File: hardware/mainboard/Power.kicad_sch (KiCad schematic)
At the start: 49 parts, among them IC1 3.3V/0.5A, IC2 TPS54202HDDCR, U12 LMR33640DDDA

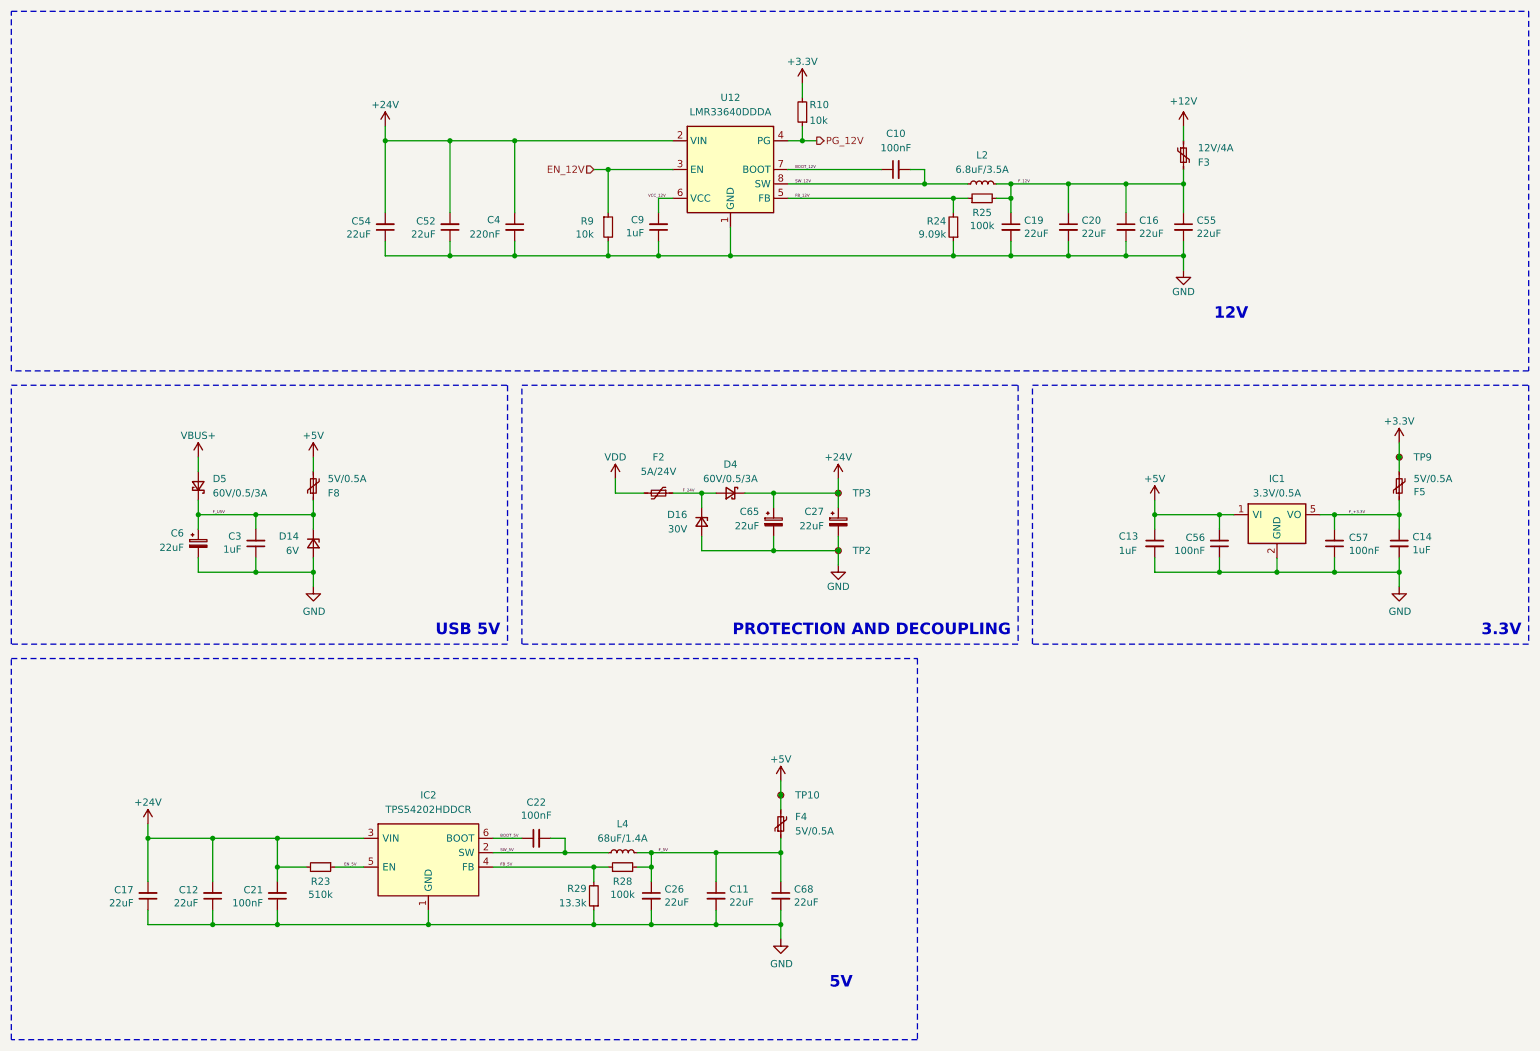
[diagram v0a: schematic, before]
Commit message: sync
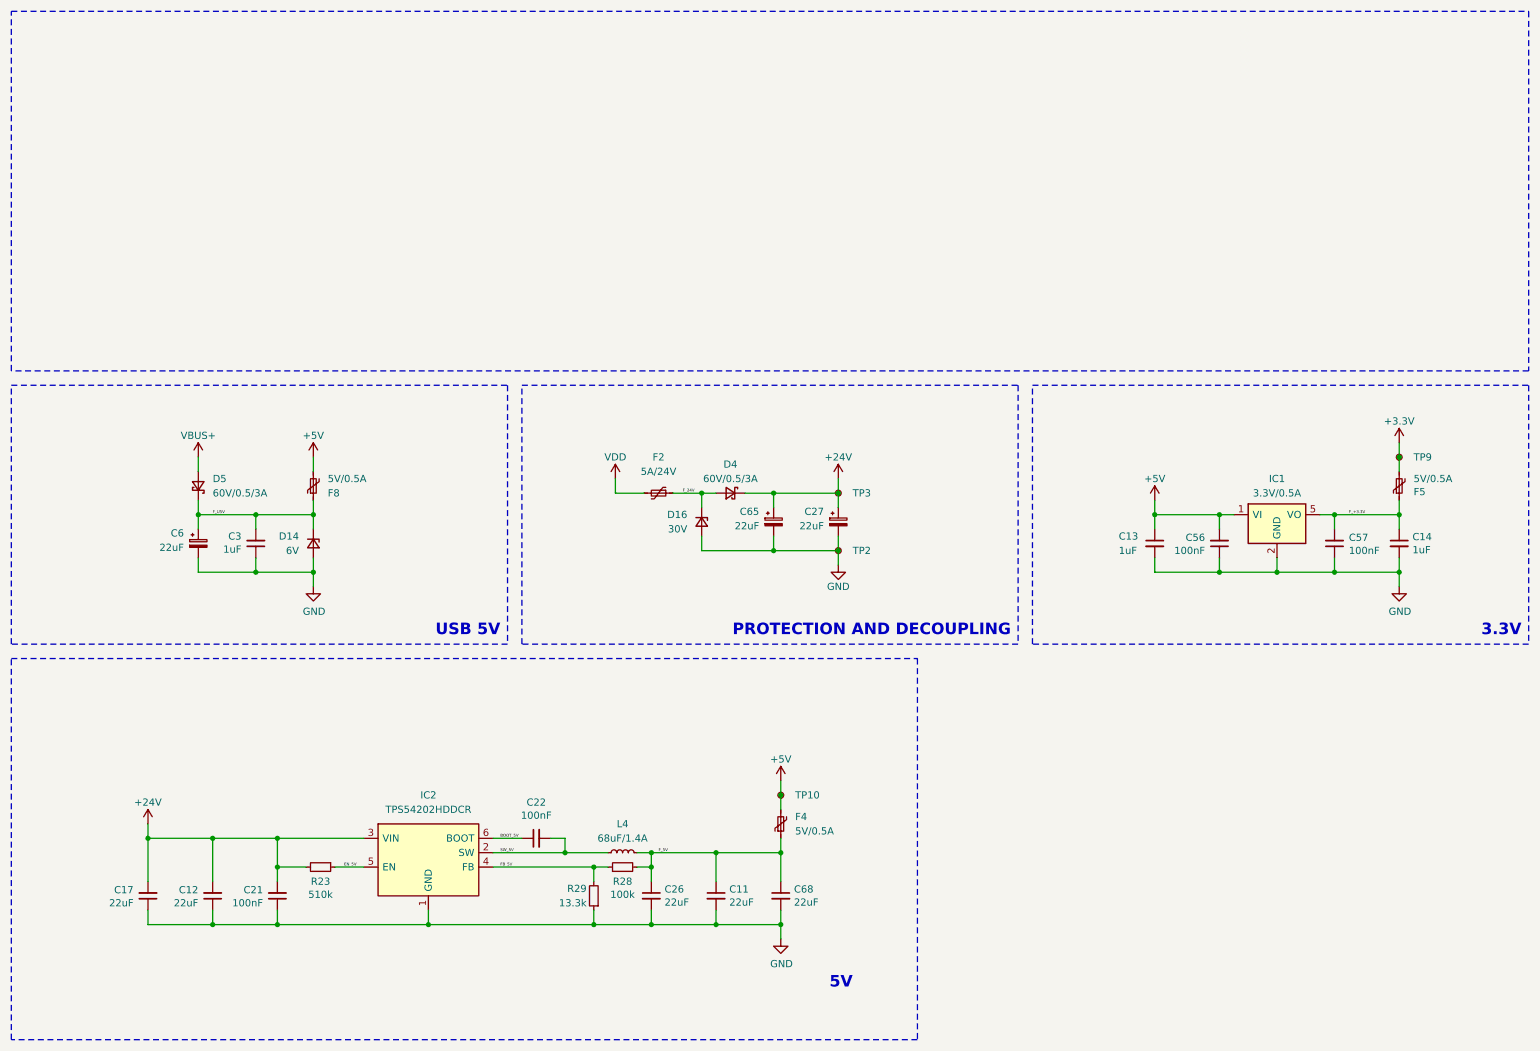
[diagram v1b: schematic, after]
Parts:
- removed C10: 100nF, Capacitor_SMD:C_0603_1608Metric, symbol Device:C_Small
- removed C16, C19, C20, C52, C54, C55: 22uF, Capacitor_SMD:C_0805_2012Metric, symbol Device:C_Small
- removed C4: 220nF, Capacitor_SMD:C_0603_1608Metric, symbol Device:C_Small
- removed C9: 1uF, Capacitor_SMD:C_0603_1608Metric, symbol Device:C_Small
- removed F3: 12V/4A, Fuse:Fuse_1206_3216Metric, symbol Device:Polyfuse_Small
- removed L2: 6.8uF/3.5A, Inductor_SMD:L_TDK_VLS6045EX_VLS6045AF, symbol Samacsys_kicad_sym:SRR4028-271Y
- removed R10, R9: 10k, Resistor_SMD:R_0603_1608Metric, symbol Device:R_Small
- removed R24: 9.09k, Resistor_SMD:R_0603_1608Metric, symbol Device:R_Small
- removed R25: 100k, Resistor_SMD:R_0603_1608Metric, symbol Device:R_Small
- removed U12: LMR33640DDDA, Package_SO:Texas_HSOP-8-1EP_3.9x4.9mm_P1.27mm, symbol Regulator_Switching:LMR33640DDDA
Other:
- note removed: "12V"

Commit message: schematic?
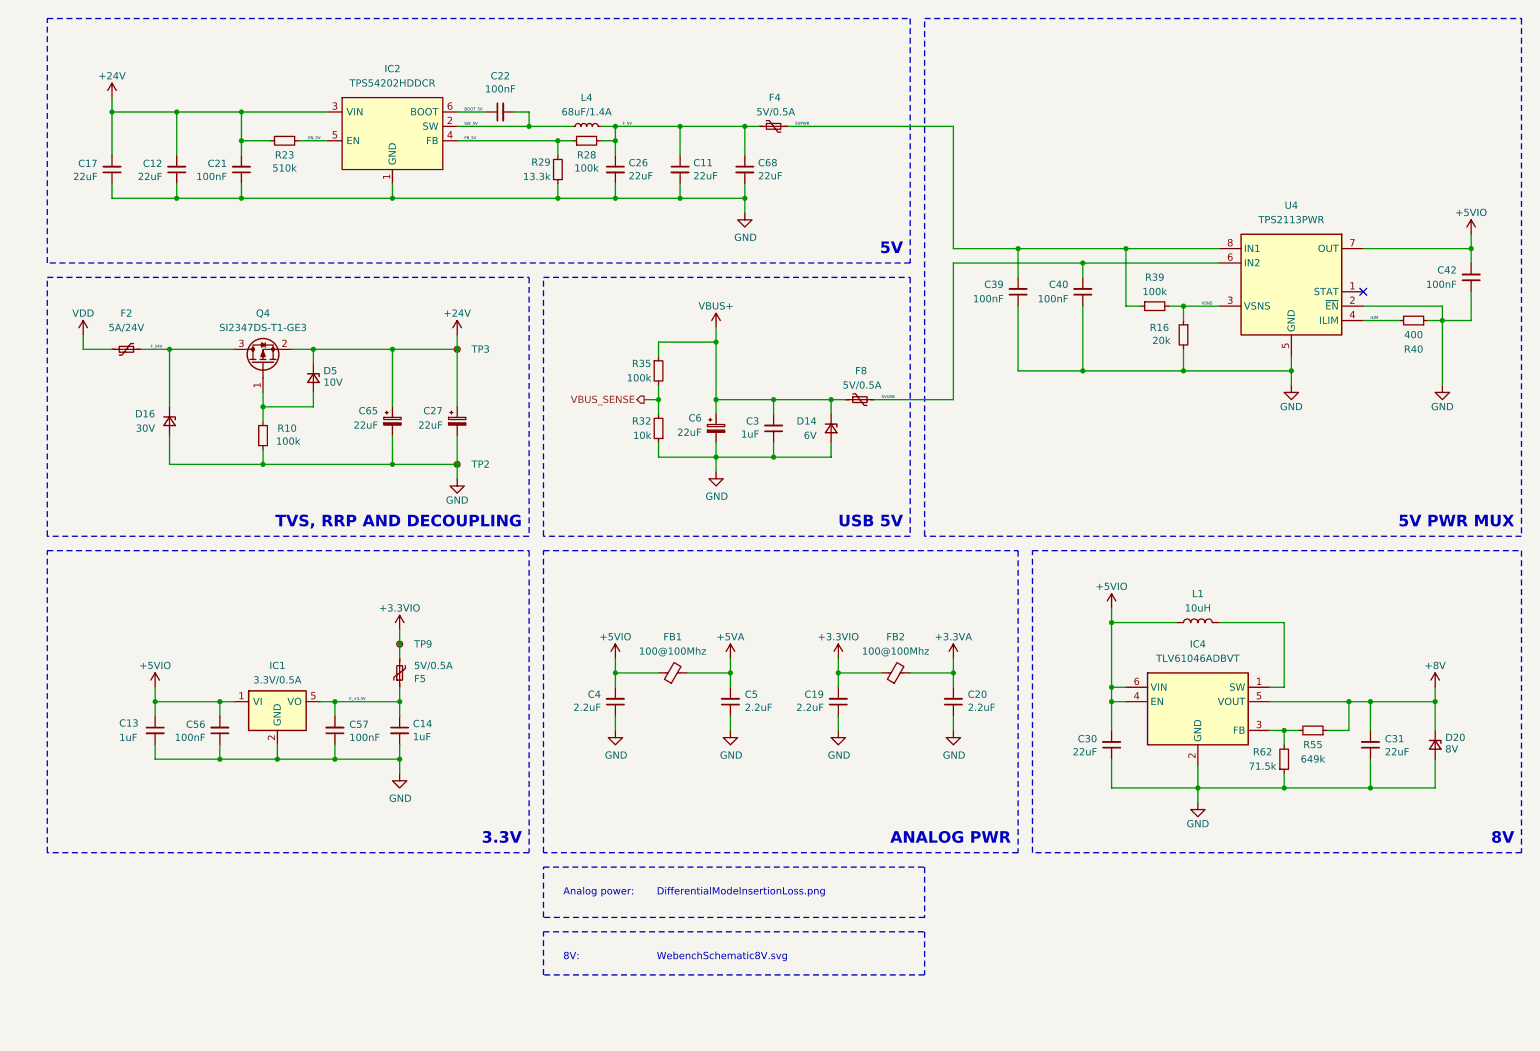
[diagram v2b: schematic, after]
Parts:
- removed D4, D5: 60V/0.5/3A, Diode_SMD:D_SOD-123, symbol Device:D_Schottky_Small
- removed TP10: TestPoint_Small, TestPoint:TestPoint_THTPad_D1.0mm_Drill0.5mm, symbol Connector:TestPoint_Small
- added C19, C20, C4, C5: 2.2uF, Capacitor_SMD:C_0603_1608Metric, symbol Device:C_Small
- added C30, C31: 22uF, Capacitor_SMD:C_0805_2012Metric, symbol Device:C_Small
- added C39, C40, C42: 100nF, Capacitor_SMD:C_0603_1608Metric, symbol Device:C_Small
- added D20: 8V, Diode_SMD:D_SOD-123, symbol Device:D_Zener_Small
- added D5: 10V, Diode_SMD:D_SOD-123, symbol Device:D_Zener_Small
- added FB1, FB2: 100@100Mhz, Inductor_SMD:L_0603_1608Metric, symbol Device:FerriteBead_Small
- added IC4: TLV61046ADBVT, Package_TO_SOT_SMD:SOT-23-6, symbol Samacsys_kicad_sym:TLV61046ADBVT
- added L1: 10uH, Inductor_SMD:L_1008_2520Metric, symbol Device:L
- added Q4: SI2347DS-T1-GE3, Package_TO_SOT_SMD:SOT-23-3, symbol Transistor_FET:Q_PMOS_GSD
- added R10: 100k, Resistor_SMD:R_0603_1608Metric_Pad0.98x0.95mm_HandSolder, symbol Device:R_Small
- added R16: 20k, Resistor_SMD:R_0603_1608Metric, symbol Device:R_Small
- added R32: 10k, Resistor_SMD:R_0603_1608Metric, symbol Device:R_Small
- added R35, R39: 100k, Resistor_SMD:R_0603_1608Metric, symbol Device:R_Small
- added R40: 400, Resistor_SMD:R_0603_1608Metric, symbol Device:R_Small
- added R55: 649k, Resistor_SMD:R_0603_1608Metric, symbol Device:R_Small
- added R62: 71.5k, Resistor_SMD:R_0603_1608Metric, symbol Device:R_Small
- added U4: TPS2113PWR, Package_SO:TSSOP-8_4.4x3mm_P0.65mm, symbol Samacsys_kicad_sym:TPS2113PWR
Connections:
- net F_U5V is gone; now on net VBUS+: C3.2, C6.1, D14.1 (K), F8.1
- net +24V: now also D5.1 (K), Q4.2 (S)
- net F_24V: now also Q4.3 (D)
- net GND: now also C19.1, C20.1, C30.1, C31.1, C39.1, C4.1, C40.1, C42.1, C5.1, D20.2 (A), IC4.2 (GND), R10.2, R16.2, R32.1, R40.1, R62.1, U4.2 (~{EN}), U4.5 (GND)
- net VBUS+: now also R35.1
- net +3.3V renamed +3.3VIO
- net +3.3VIO: now also C19.2, FB2.1
- net +5V renamed +5VIO
- net +5VIO: now also C30.2, C4.2, C42.2, FB1.1, IC4.4 (EN), IC4.6 (VIN), L1.1, U4.7 (OUT); no longer F4.2, F8.2
- new net: D5.2 (A), Q4.1 (G), R10.1
- new net: IC4.3 (FB), R55.2, R62.2
- new net: IC4.1 (SW), L1.2
- new net +3.3VA: C20.2, FB2.2
- new net +5VA: C5.2, FB1.2
- new net +8V: C31.2, D20.1 (K), IC4.5 (VOUT), R55.1
- new net 5VPWR: C39.2, F4.2, R39.1, U4.8 (IN1)
- new net 5VUSB: C40.2, F8.2, U4.6 (IN2)
- new net ILIM: R40.2, U4.4 (ILIM)
- new net VBUS_SENSE: R32.2, R35.2
- new net VSNS: R16.1, R39.2, U4.3 (VSNS)
- no-connect marks 0 -> 1
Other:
- note added: "5V PWR MUX"
- note added: "8V"
- note added: "ANALOG PWR"
- note added: "TVS, RRP AND DECOUPLING"
- note removed: "PROTECTION AND DECOUPLING"
- moved on the sheet: C11, C12, C13, C14, C17, C21, C22, C26, C27, C3, C56, C57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

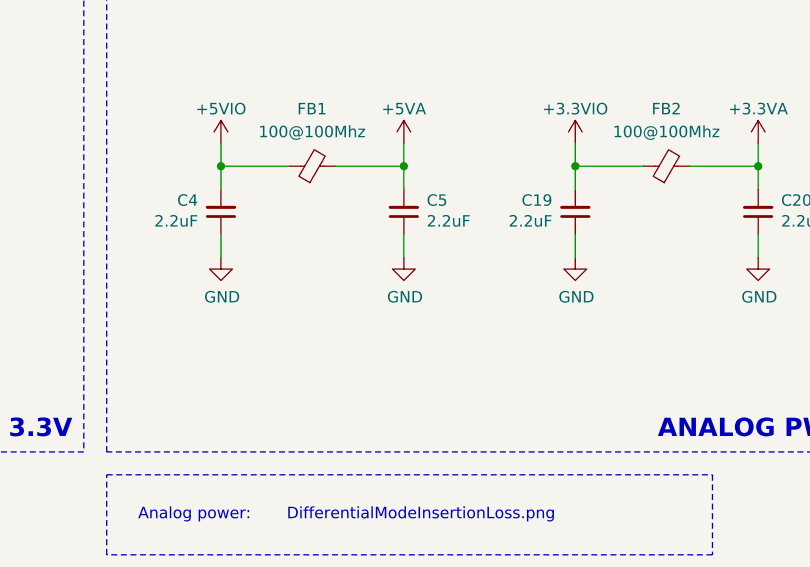
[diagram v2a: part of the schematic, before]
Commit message: v3.3
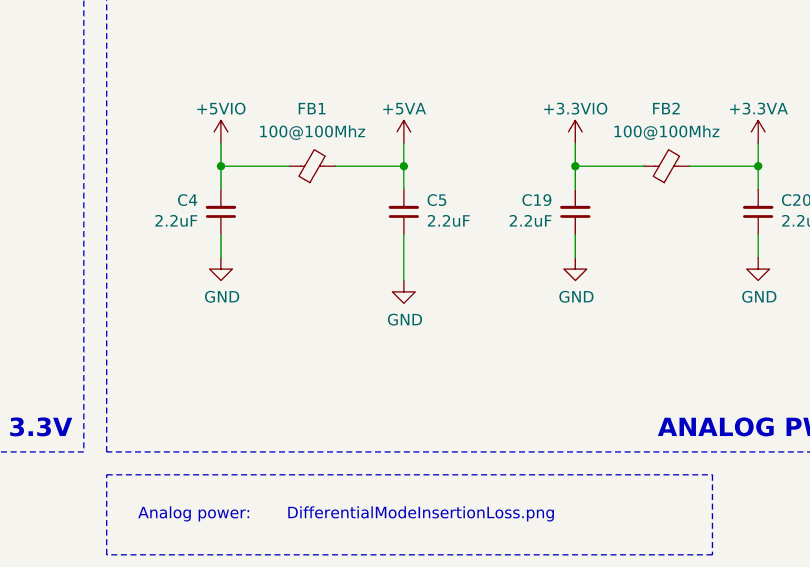
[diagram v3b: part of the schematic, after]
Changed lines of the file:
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@@
 	(wire
 		(pts
-			(xy 140.97 138.43) (xy 140.97 140.97)
-		)
-		(stroke
-			(width 0)
-			(type default)
-		)
-	)
-	(wire
-		(pts
 			(xy 110.49 46.99) (xy 110.49 44.45)
 		)
@@
 	(wire
 		(pts
+			(xy 140.97 138.43) (xy 140.97 143.51)
+		)
+		(stroke
+			(width 0)
+			(type default)
+		)
+	)
+	(wire
+		(pts
 			(xy 160.02 138.43) (xy 160.02 140.97)
 		)
@@
 		(lib_name "GND_2")
 		(lib_id "power:GND")
-		(at 140.97 140.97 0)
+		(at 140.97 143.51 0)
 		(unit 1)
 		(exclude_from_sim no)
@@
 		(dnp no)
 		(property "Reference" "#PWR07"
-			(at 140.97 147.32 0)
+			(at 140.97 149.86 0)
 			(effects
 				(font
@@
 		)
 		(property "Value" "GND"
-			(at 141.097 145.3642 0)
+			(at 141.097 147.9042 0)
 			(effects
 				(font
@@
 		)
 		(property "Footprint" ""
-			(at 140.97 140.97 0)
+			(at 140.97 143.51 0)
 			(effects
 				(font
@@
 		)
 		(property "Datasheet" ""
-			(at 140.97 140.97 0)
+			(at 140.97 143.51 0)
 			(effects
 				(font
@@
 		)
 		(property "Description" ""
-			(at 140.97 140.97 0)
+			(at 140.97 143.51 0)
 			(effects
 				(font
